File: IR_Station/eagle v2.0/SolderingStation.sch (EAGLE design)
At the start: 112 parts, among them IC1 LM317, J1 JP4, J2 JP4, J3 JP4, J4 JP4, U1 MSP340G2443, U2 UPD166010, U3 MCP6V08, U4 UPD166010, U5 MCP6V08, U6 ADS1115IDGST

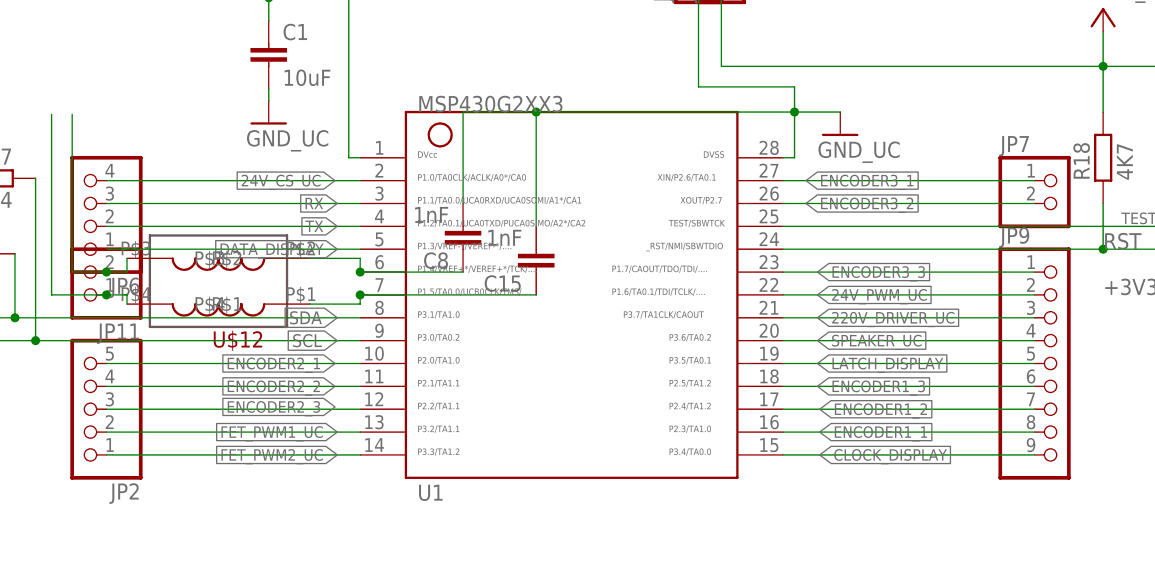
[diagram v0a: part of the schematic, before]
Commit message: 04.04.2018
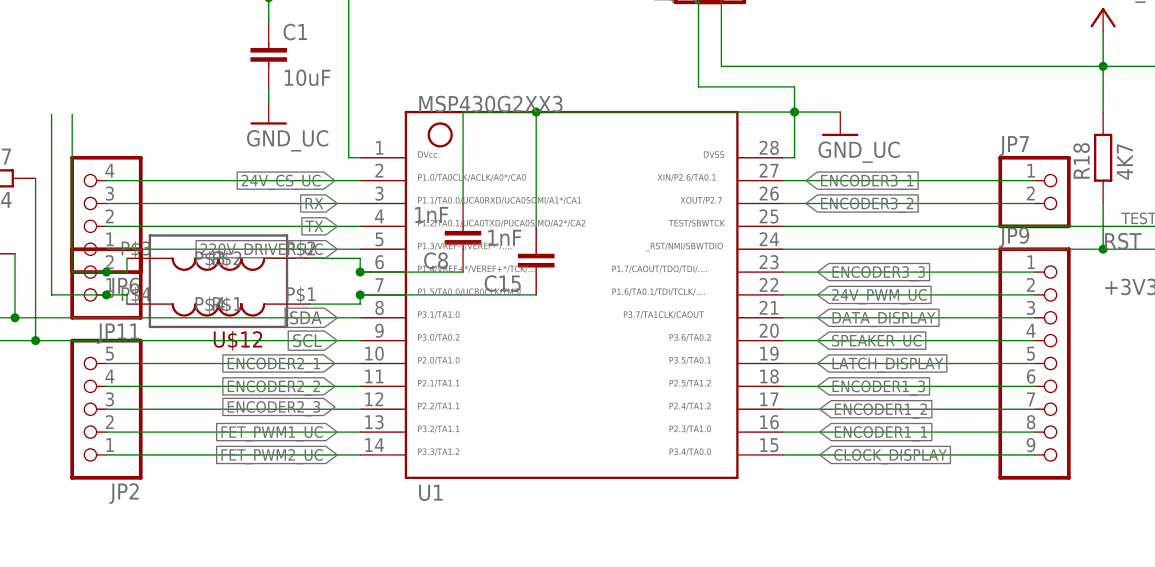
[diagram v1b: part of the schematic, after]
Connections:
- net 220V_DRIVER_UC: now also JP6.1, U1.5; no longer JP9.3, U1.21
- net DATA_DISPLAY: now also JP9.3, U1.21; no longer JP6.1, U1.5
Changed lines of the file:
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@@
-</segment>
-</net>
-<net name="DATA_DISPLAY" class="0">
-<segment>
-<pinref part="U1" gate="G$1" pin="5"/>
-<label x="176.53" y="48.514" size="1.27" layer="95" rot="R180" xref="yes"/>
-<wire x1="179.07" y1="48.514" x2="150.876" y2="48.514" width="0.1524" layer="91"/>
-<pinref part="JP6" gate="A" pin="1"/>
 </segment>
 </net>
@@
 <net name="220V_DRIVER_UC" class="0">
 <segment>
-<pinref part="U1" gate="G$1" pin="21"/>
-<label x="229.87" y="40.894" size="1.27" layer="95" xref="yes"/>
-<wire x1="226.06" y1="40.894" x2="254" y2="40.894" width="0.1524" layer="91"/>
-<pinref part="JP9" gate="A" pin="3"/>
+<pinref part="U1" gate="G$1" pin="5"/>
+<label x="176.53" y="48.514" size="1.27" layer="95" rot="R180" xref="yes"/>
+<wire x1="179.07" y1="48.514" x2="150.876" y2="48.514" width="0.1524" layer="91"/>
+<pinref part="JP6" gate="A" pin="1"/>
 </segment>
 </net>
@@
 </segment>
 </net>
+<net name="DATA_DISPLAY" class="0">
+<segment>
+<pinref part="U1" gate="G$1" pin="21"/>
+<label x="229.87" y="40.894" size="1.27" layer="95" xref="yes"/>
+<wire x1="226.06" y1="40.894" x2="254" y2="40.894" width="0.1524" layer="91"/>
+<pinref part="JP9" gate="A" pin="3"/>
+</segment>
+</net>
